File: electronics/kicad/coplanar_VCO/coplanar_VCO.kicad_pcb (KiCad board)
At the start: 2 copper layers, 38 parts, among them J1 CONN_01, J2 CONN_01, P1 a, P4 a, P5 a, P6 a, P7 a, P8 a, U2 HMC732, U7 CE3520K3

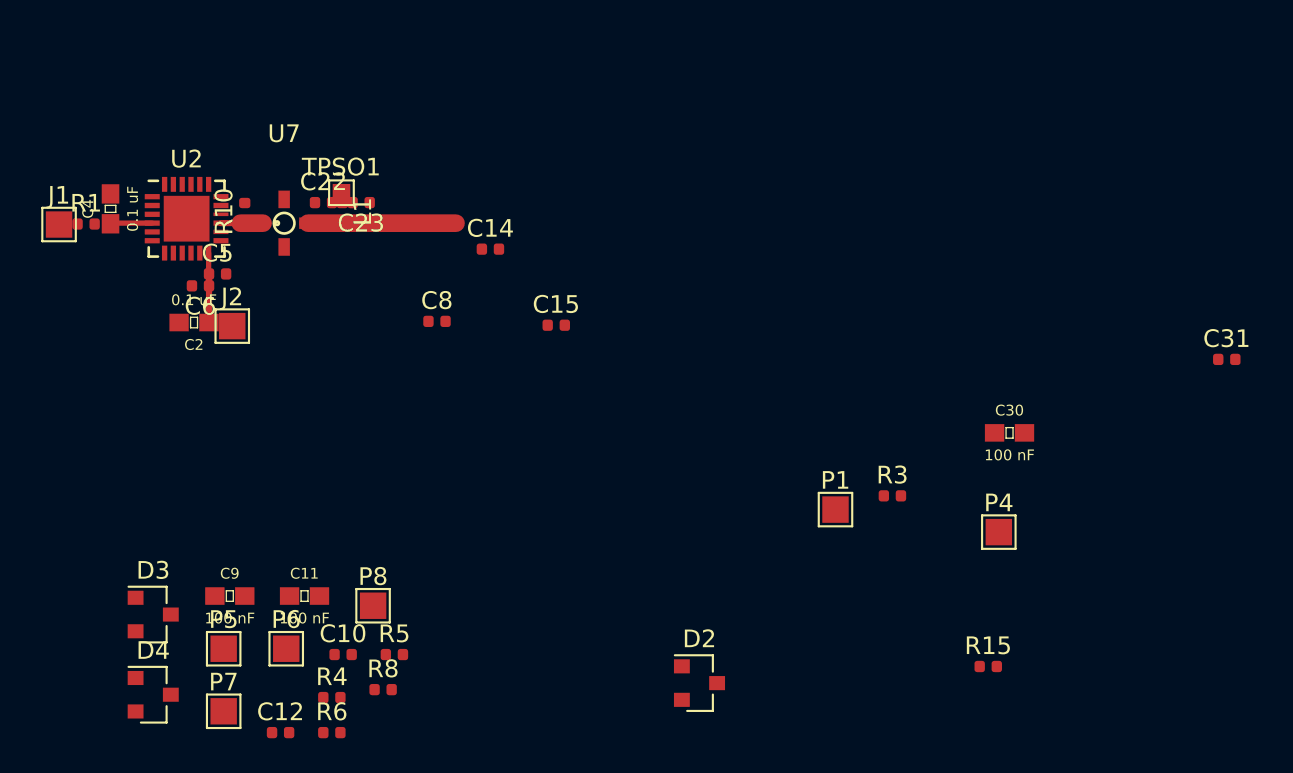
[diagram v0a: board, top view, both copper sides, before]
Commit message: Coplanar
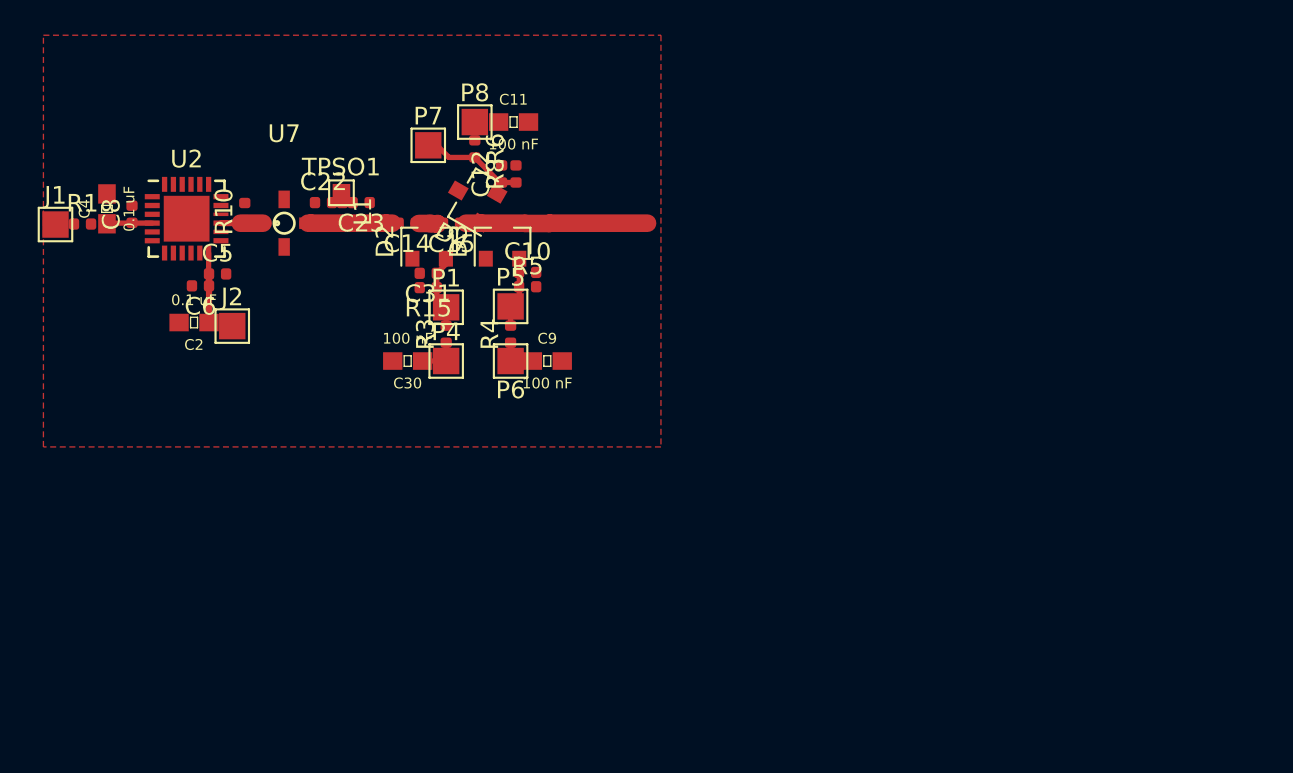
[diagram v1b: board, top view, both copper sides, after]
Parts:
- moved C31 45.6 mm to (36.6, 23.7), turned to 180 degrees
- moved R15 38.4 mm to (36.6, 24.5), turned to 180 degrees
- moved C30 34.4 mm to (35.4, 28.7), turned to 180 degrees
- moved P7 34.2 mm to (36.6, 16.4)
- moved R6 34.1 mm to (39.2, 16.6), turned to 270 degrees
- moved C12 34.1 mm to (40.7, 18.0), turned to 90 degrees
- moved D4 33.5 mm to (39.1, 19.5), turned to 150 degrees
- moved P4 32.8 mm to (37.6, 28.7)
- moved R8 30.2 mm to (41.6, 18.0), turned to 90 degrees
- moved D2 29.4 mm to (36.6, 21.8), turned to 90 degrees
- moved C11 29.4 mm to (41.4, 15.1)
- moved D3 29.0 mm to (40.8, 21.8), turned to 90 degrees
- moved P8 28.1 mm to (39.2, 15.1)
- moved R3 26.9 mm to (37.6, 27.1), turned to 90 degrees
- moved P5 25.4 mm to (41.2, 25.6)
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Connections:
- U2 pad 10: (no net) -> GND
- U2 pad 11: (no net) -> GND
- U2 pad 13: (no net) -> GND
- U2 pad 16: (no net) -> GND
- U2 pad 17: (no net) -> GND
- U2 pad 18: (no net) -> GND
- U2 pad 19: (no net) -> GND
- U2 pad 20: (no net) -> GND
- U2 pad 21: (no net) -> GND
- U2 pad 22: (no net) -> GND
- U2 pad 5: (no net) -> GND
- U2 pad 6: (no net) -> GND
- U2 pad 7: (no net) -> GND
- U2 pad 8: (no net) -> GND
- U2 pad 9: (no net) -> GND
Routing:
- net Net-(C15-Pad1): track 0.00 -> 10.3 mm
- net Net-(C12-Pad1): track 0.00 -> 7.15 mm
- net Net-(C31-Pad1): track 0.00 -> 4.23 mm
- net Net-(C10-Pad1): track 0.00 -> 4.00 mm
- net Net-(C14-Pad2): track 8.40 -> 4.80 mm
- net Net-(C30-Pad1): track 0.00 -> 2.38 mm
- net Net-(C9-Pad1): track 0.00 -> 2.27 mm
- net Net-(C14-Pad1): track 0.00 -> 1.24 mm
- added copper zone on F.Cu, net GND
